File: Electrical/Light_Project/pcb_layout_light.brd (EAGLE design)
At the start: 30.5 x 23.8 mm, 6 parts, among them U1 REG710NA-3.3/3K, U2 ATTINY85V-10SU, U3 FSM8JRT

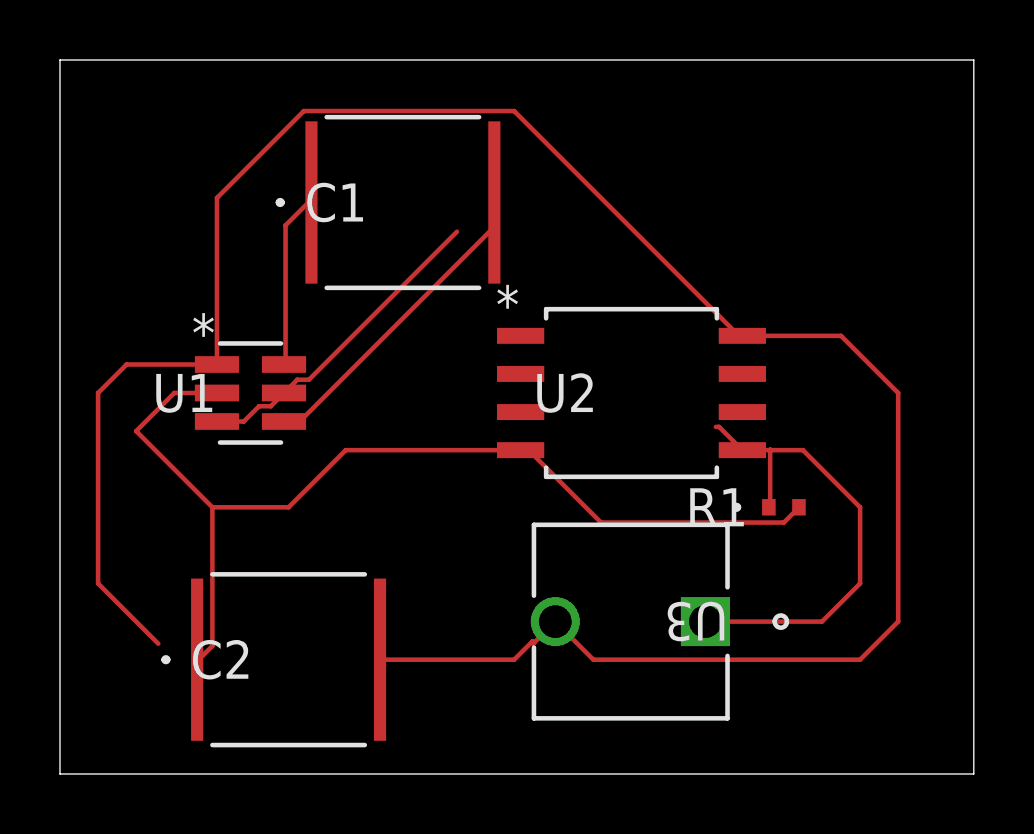
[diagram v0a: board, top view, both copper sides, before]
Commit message: add pdf of new layout
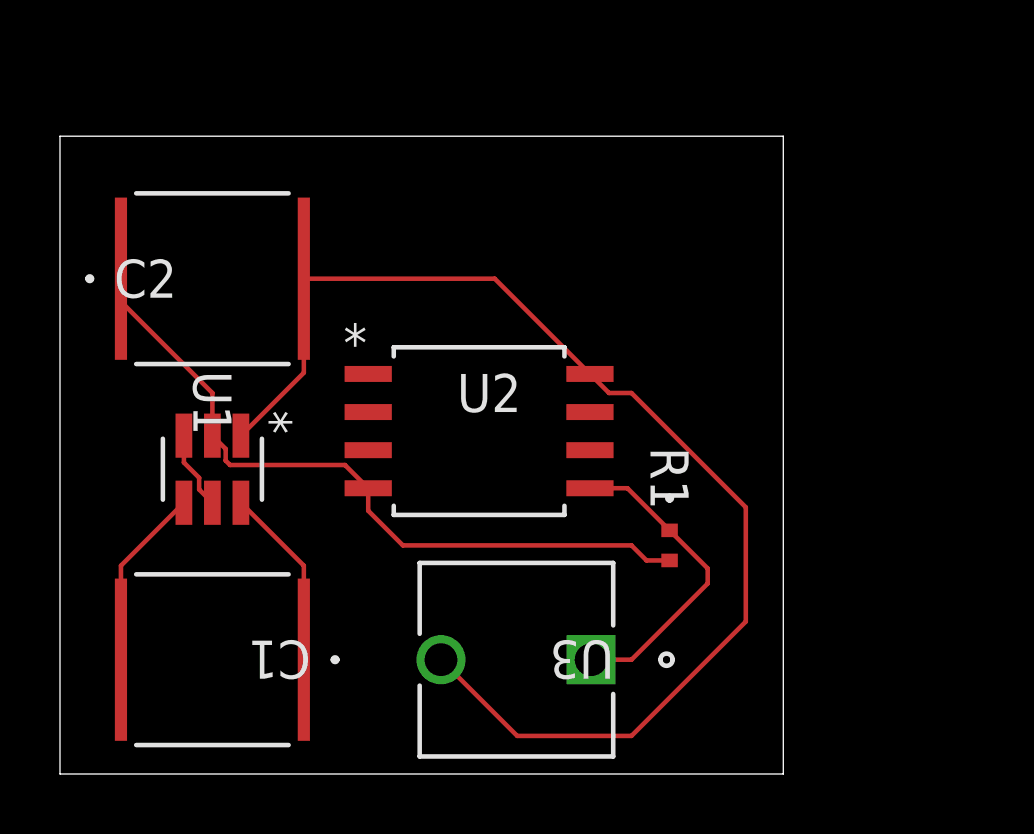
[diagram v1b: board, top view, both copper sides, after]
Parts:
- moved C1 16.5 mm to (30.5, 3.81), turned to 180 degrees
- moved C2 13.0 mm to (30.5, 16.5)
- moved U2 5.24 mm to (39.4, 11.4)
- moved R1 4.02 mm to (45.7, 7.62), turned to 270 degrees
- moved U3 4.02 mm to (38.1, 3.81)
- moved U1 2.84 mm to (30.5, 10.2), turned to 270 degrees
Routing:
- net N$1: track 73.4 -> 40.6 mm
- net GND: track 33.9 -> 24.6 mm
- net N$4: track 10.6 -> 2.63 mm
- net N$5: track 16.1 -> 10.5 mm
- net N$3: track 10.6 -> 6.10 mm
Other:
- board size 30.5 x 23.8 mm -> 24.1 x 21.3 mm
